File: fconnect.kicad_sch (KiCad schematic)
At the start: 192 parts, among them J1 9001-11961C00A, J2 9001-11961C00A, J3 7760, J4 7760

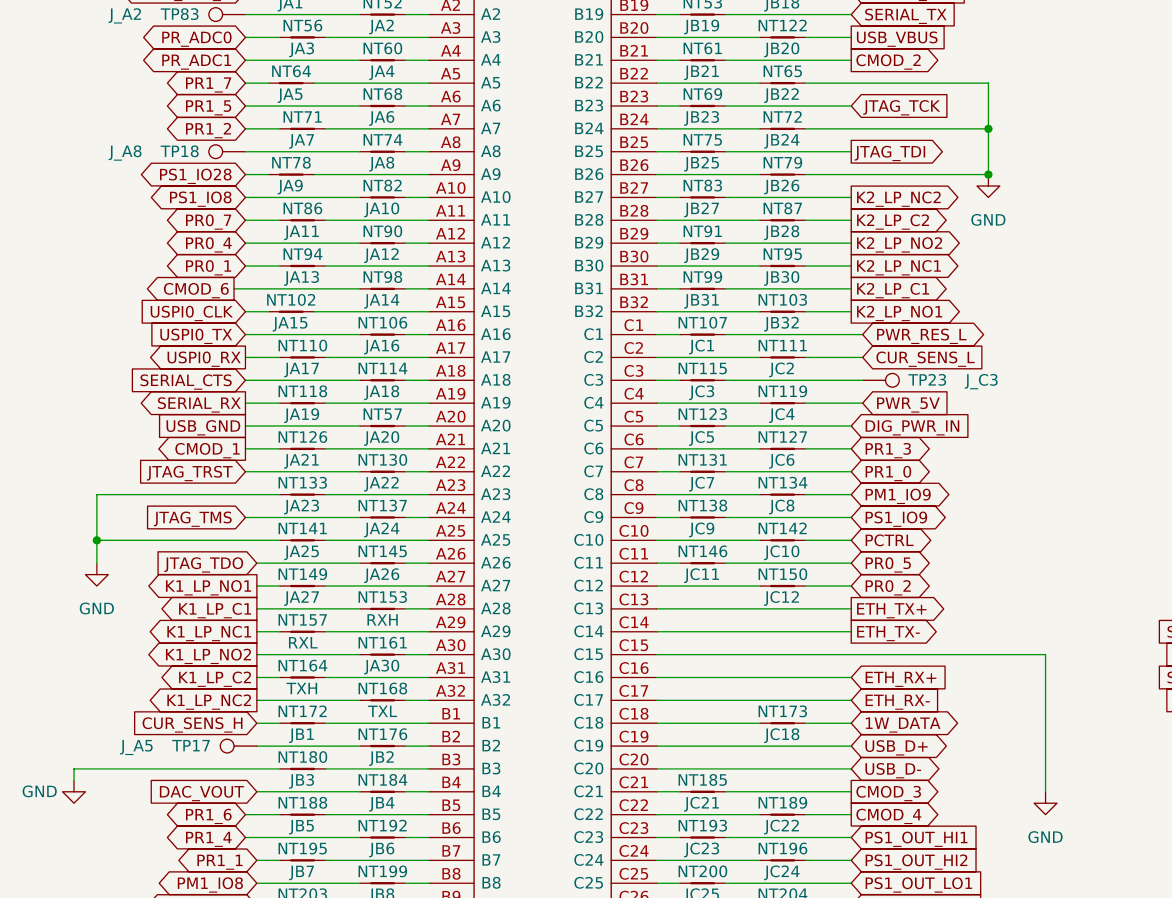
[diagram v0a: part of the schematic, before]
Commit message: update
Correction of small error
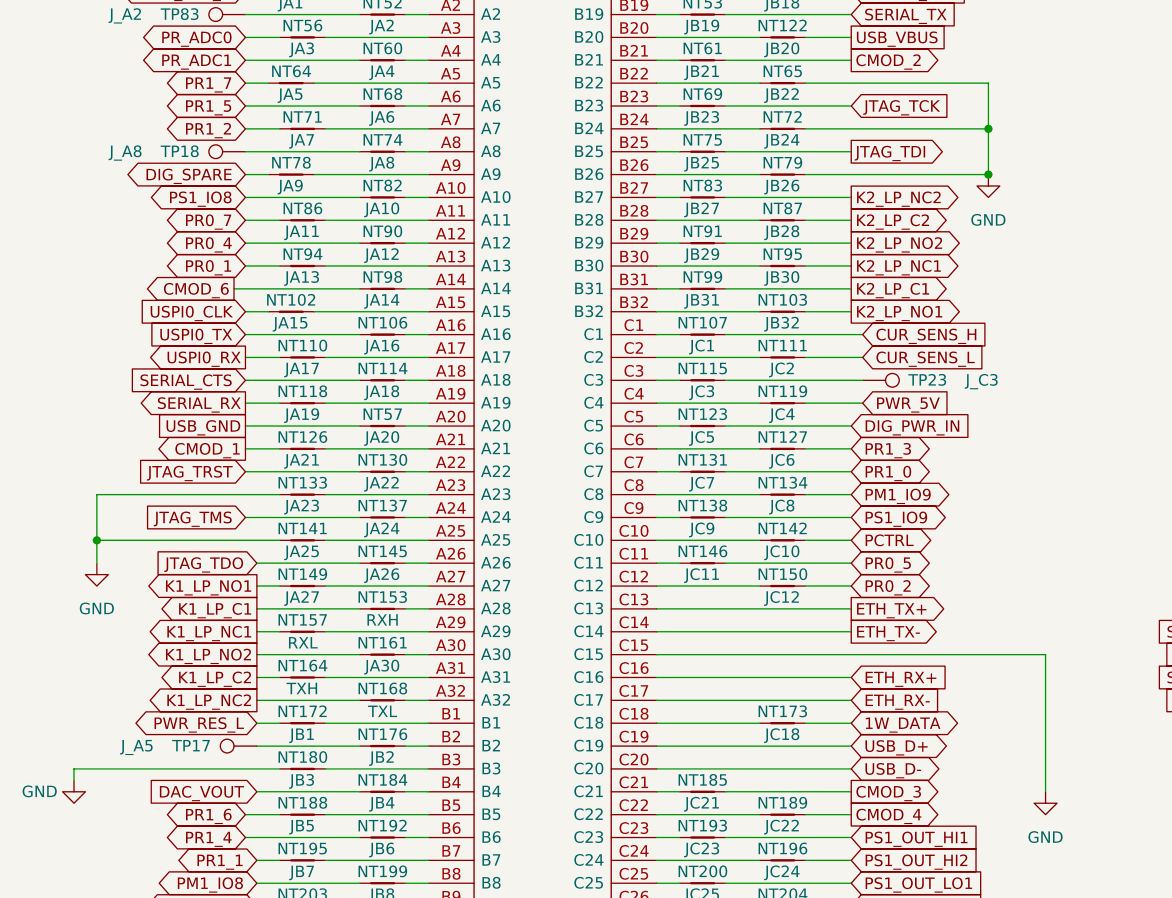
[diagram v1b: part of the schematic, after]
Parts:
- R4: footprint Resistor_THT:R_Axial_DIN0309_L9.0mm_D3.2mm_P12.70mm_Horizontal -> Resistor_THT:R_Axial_DIN0207_L6.3mm_D2.5mm_P10.16mm_Horizontal
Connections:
- net CUR_SENS_H: now also NT107.1; no longer NT172.1
- net PWR_RES_L: now also NT172.1; no longer NT107.1
- net PS1_IO28 renamed DIG_SPARE
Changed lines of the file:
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@@
     )
   )
-  (global_label "PS1_IO28" (shape bidirectional) (at 44.45 57.15 180) (fields_autoplaced)
-    (effects (font (size 1.27 1.27)) (justify right))
-    (property "Intersheet References" "${INTERSHEET_REFS}" (id 0) (at 33.0259 57.0706 0)
+  (global_label "DIG_SPARE" (shape bidirectional) (at 44.45 57.15 180) (fields_autoplaced)
+    (effects (font (size 1.27 1.27)) (justify right))
+    (property "Intersheet References" "${INTERSHEET_REFS}" (id 0) (at 31.9374 57.0706 0)
       (effects (font (size 1.27 1.27)) (justify right) hide)
     )
@@
     )
   )
-  (global_label "CUR_SENS_H" (shape input) (at 45.72 118.11 180) (fields_autoplaced)
-    (effects (font (size 1.27 1.27)) (justify right))
-    (property "Intersheet References" "${INTERSHEET_REFS}" (id 0) (at 31.2721 118.0306 0)
-      (effects (font (size 1.27 1.27)) (justify right) hide)
-    )
-  )
   (global_label "PR0_4" (shape bidirectional) (at 44.45 64.77 180) (fields_autoplaced)
     (effects (font (size 1.27 1.27)) (justify right))
@@
     )
   )
-  (global_label "PWR_RES_L" (shape bidirectional) (at 113.03 74.93 0) (fields_autoplaced)
-    (effects (font (size 1.27 1.27)) (justify left))
-    (property "Intersheet References" "${INTERSHEET_REFS}" (id 0) (at 126.0264 74.8506 0)
-      (effects (font (size 1.27 1.27)) (justify left) hide)
-    )
-  )
   (global_label "B33_H" (shape input) (at 160.02 72.39 180) (fields_autoplaced)
     (effects (font (size 1.27 1.27)) (justify right))
@@
     )
   )
+  (global_label "CUR_SENS_H" (shape input) (at 113.03 74.93 0) (fields_autoplaced)
+    (effects (font (size 1.27 1.27)) (justify left))
+    (property "Intersheet References" "${INTERSHEET_REFS}" (id 0) (at 127.4779 74.8506 0)
+      (effects (font (size 1.27 1.27)) (justify left) hide)
+    )
+  )
   (global_label "K1_LP_C2" (shape output) (at 45.72 113.03 180) (fields_autoplaced)
     (effects (font (size 1.27 1.27)) (justify right))
@@
     (property "Intersheet References" "${INTERSHEET_REFS}" (id 0) (at 123.8493 41.9894 0)
       (effects (font (size 1.27 1.27)) (justify left) hide)
+    )
+  )
+  (global_label "PWR_RES_L" (shape bidirectional) (at 45.72 118.11 180) (fields_autoplaced)
+    (effects (font (size 1.27 1.27)) (justify right))
+    (property "Intersheet References" "${INTERSHEET_REFS}" (id 0) (at 32.7236 118.0306 0)
+      (effects (font (size 1.27 1.27)) (justify right) hide)
     )
   )
@@
     (property "Reference" "R4" (id 0) (at 49.53 190.5 0))
     (property "Value" "0" (id 1) (at 58.42 190.5 0))
-    (property "Footprint" "Resistor_THT:R_Axial_DIN0309_L9.0mm_D3.2mm_P12.70mm_Horizontal" (id 2) (at 53.594 188.976 90)
-      (effects (font (size 1.27 1.27)) hide)
-    )
+    (property "Footprint" "Resistor_THT:R_Axial_DIN0207_L6.3mm_D2.5mm_P10.16mm_Horizontal" (id 2) (at 53.594 188.976 90)
+      (effects (font (size 1.27 1.27)) hide)
+    )
